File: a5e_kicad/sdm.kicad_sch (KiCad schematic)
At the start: 25 parts, among them U6 MT25QU256ABB8E12-0SIT, U7 A5EB013B-B23B

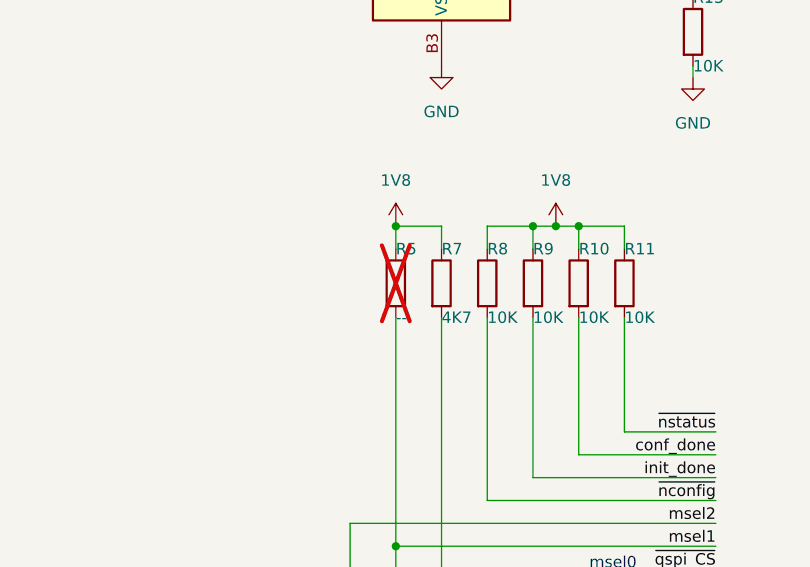
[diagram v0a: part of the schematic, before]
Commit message: savegame, after fixing wird problems with schematic sync
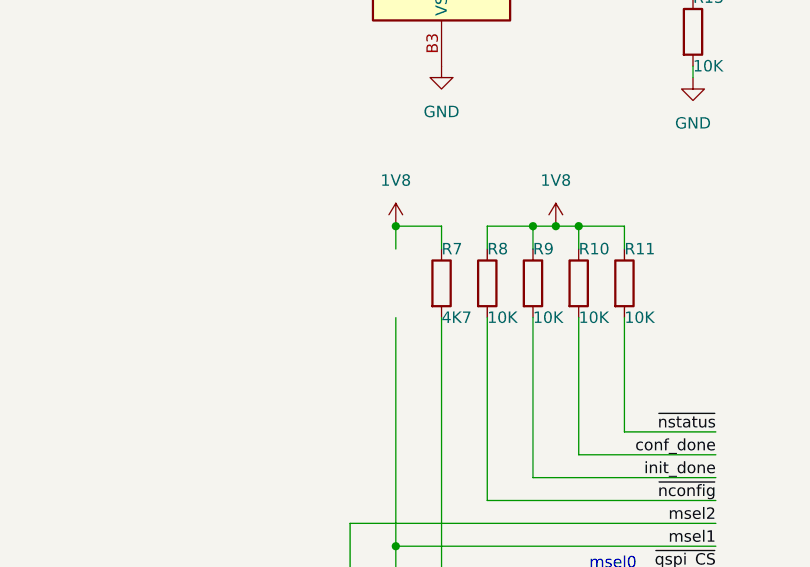
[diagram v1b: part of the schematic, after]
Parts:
- removed R5: --, Resistor_SMD:R_0402_1005Metric, symbol Device:R
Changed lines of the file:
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@@
-	)
-	(symbol
-		(lib_id "Device:R")
-		(at 53.34 105.41 0)
-		(unit 1)
-		(body_style 1)
-		(exclude_from_sim no)
-		(in_bom no)
-		(on_board yes)
-		(in_pos_files yes)
-		(dnp yes)
-		(property "Reference" "R5"
-			(at 53.34 101.6 0)
-			(show_name no)
-			(do_not_autoplace no)
-			(effects
-				(font
-					(size 1.27 1.27)
-				)
-				(justify left)
-			)
-		)
-		(property "Value" "--"
-			(at 53.34 109.22 0)
-			(show_name no)
-			(do_not_autoplace no)
-			(effects
-				(font
-					(size 1.27 1.27)
-				)
-				(justify left)
-			)
-		)
-		(property "Footprint" "Resistor_SMD:R_0402_1005Metric"
-			(at 51.562 105.41 90)
-			(hide yes)
-			(show_name no)
-			(do_not_autoplace no)
-			(effects
-				(font
-					(size 1.27 1.27)
-				)
-			)
-		)
-		(property "Datasheet" ""
-			(at 53.34 105.41 0)
-			(hide yes)
-			(show_name no)
-			(do_not_autoplace no)
-			(effects
-				(font
-					(size 1.27 1.27)
-				)
-			)
-		)
-		(property "Description" "Resistor"
-			(at 53.34 105.41 0)
-			(hide yes)
-			(show_name no)
-			(do_not_autoplace no)
-			(effects
-				(font
-					(size 1.27 1.27)
-				)
-			)
-		)
-		(pin "2"
-		)
-		(pin "1"
-		)
-		(instances
-			(project "DBM_A5E013"
-				(path "/267d02d2-570f-41a1-8015-b378cedbc665/8aaf6c2b-ae6e-4499-806d-67948f95803c"
-					(reference "R203")
-					(unit 1)
-				)
-			)
-			(project "agilex_3_soc"
-				(path "/a5b98d95-6877-4284-904f-d04e32723ae0/8aaf6c2b-ae6e-4499-806d-67948f95803c"
-					(reference "R5")
-					(unit 1)
-				)
-			)
-		)
 	)
 	(symbol
